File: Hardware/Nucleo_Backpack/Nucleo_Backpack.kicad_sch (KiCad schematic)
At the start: 9 parts, among them J1 CN7, J2 CN10, J4 Conn_01x04

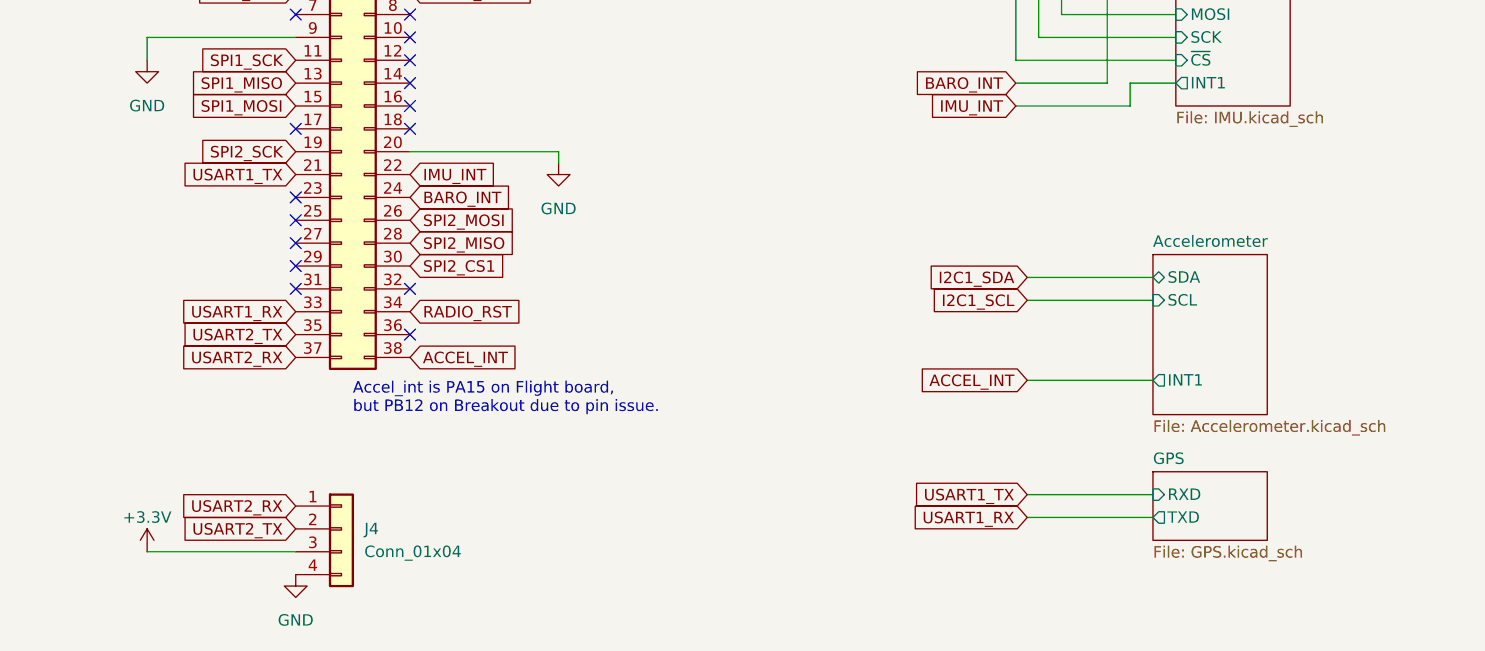
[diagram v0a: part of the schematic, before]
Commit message: Backpack Updates
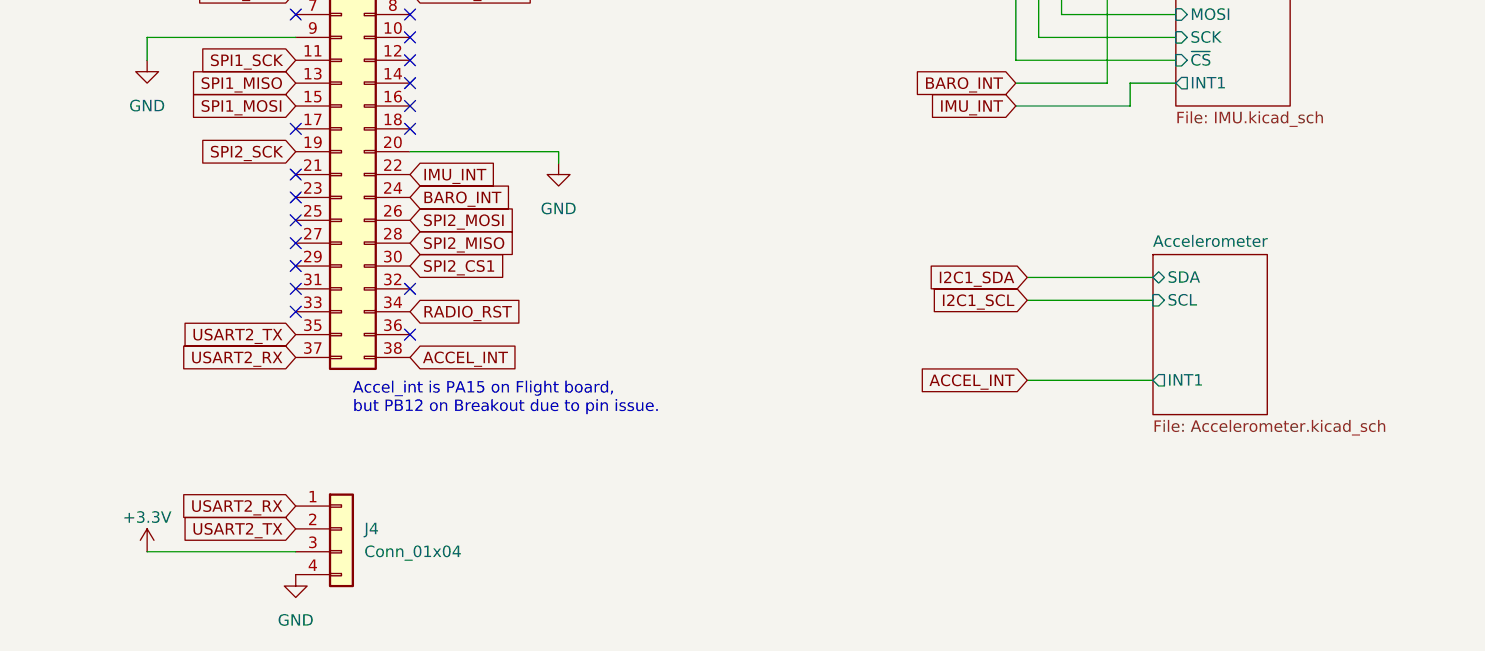
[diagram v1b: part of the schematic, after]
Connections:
- net USART1_RX: no longer names the net of J2.33 (Pin_33)
- net USART1_TX: no longer names the net of J2.21 (Pin_21)
- no-connect marks 39 -> 41
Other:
- removed sheet GPS
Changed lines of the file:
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@@
   (no_connect (at 106.68 110.49))
   (no_connect (at 181.61 91.44))
+  (no_connect (at 168.91 109.22))
   (no_connect (at 106.68 118.11))
   (no_connect (at 106.68 92.71))
@@
   (no_connect (at 181.61 99.06))
   (no_connect (at 181.61 127))
+  (no_connect (at 168.91 124.46))
   (wire (pts (xy 250.19 132.08) (xy 264.16 132.08))
     (stroke (width 0) (type default))
   )
-  (wire (pts (xy 250.19 144.78) (xy 264.16 144.78))
-    (stroke (width 0) (type default))
-  )
   (wire (pts (xy 248.92 73.66) (xy 248.92 96.52))
     (stroke (width 0) (type default))
@@
   )
   (wire (pts (xy 210.82 60.96) (xy 210.82 63.5))
-    (stroke (width 0) (type default))
-  )
-  (wire (pts (xy 250.19 147.32) (xy 264.16 147.32))
     (stroke (width 0) (type default))
   )
@@
     )
   )
-  (global_label "USART1_RX" (shape input) (at 250.19 147.32 180) (fields_autoplaced)
-    (effects (font (size 1.27 1.27)) (justify right))
-    (property "Intersheetrefs" "${INTERSHEET_REFS}" (at 236.5869 147.32 0)
-      (effects (font (size 1.27 1.27)) (justify right) hide)
-    )
-  )
   (global_label "BARO_INT" (shape input) (at 181.61 111.76 0) (fields_autoplaced)
     (effects (font (size 1.27 1.27)) (justify left))
@@
     )
   )
-  (global_label "USART1_TX" (shape input) (at 168.91 109.22 180) (fields_autoplaced)
-    (effects (font (size 1.27 1.27)) (justify right))
-    (property "Intersheetrefs" "${INTERSHEET_REFS}" (at 155.6093 109.22 0)
-      (effects (font (size 1.27 1.27)) (justify right) hide)
-    )
-  )
   (global_label "SPI2_SCK" (shape input) (at 168.91 106.68 180) (fields_autoplaced)
     (effects (font (size 1.27 1.27)) (justify right))
@@
     )
   )
-  (global_label "USART1_TX" (shape input) (at 250.19 144.78 180) (fields_autoplaced)
-    (effects (font (size 1.27 1.27)) (justify right))
-    (property "Intersheetrefs" "${INTERSHEET_REFS}" (at 236.8893 144.78 0)
-      (effects (font (size 1.27 1.27)) (justify right) hide)
-    )
-  )
   (global_label "SDIO_D0" (shape input) (at 181.61 83.82 0) (fields_autoplaced)
     (effects (font (size 1.27 1.27)) (justify left))
@@
     (effects (font (size 1.27 1.27)) (justify right))
     (property "Intersheetrefs" "${INTERSHEET_REFS}" (at 157.0607 86.36 0)
-      (effects (font (size 1.27 1.27)) (justify right) hide)
-    )
-  )
-  (global_label "USART1_RX" (shape input) (at 168.91 124.46 180) (fields_autoplaced)
-    (effects (font (size 1.27 1.27)) (justify right))
-    (property "Intersheetrefs" "${INTERSHEET_REFS}" (at 155.3069 124.46 0)
       (effects (font (size 1.27 1.27)) (justify right) hide)
     )
@@
       )
     )
-  )
-  (sheet (at 264.16 142.24) (size 12.7 7.62) (fields_autoplaced)
-    (stroke (width 0.1524) (type solid))
-    (fill (color 0 0 0 0.0000))
-    (property "Sheetname" "GPS" (at 264.16 141.5284 0)
-      (effects (font (size 1.27 1.27)) (justify left bottom))
-    )
-    (property "Sheetfile" "GPS.kicad_sch" (at 264.16 150.4446 0)
-      (effects (font (size 1.27 1.27)) (justify left top))
-    )
-    (pin "RXD" input (at 264.16 144.78 180)
-      (effects (font (size 1.27 1.27)) (justify left))
-    )
-    (pin "TXD" output (at 264.16 147.32 180)
-      (effects (font (size 1.27 1.27)) (justify left))
-    )
-    (instances
-      (project "Nucleo_Backpack"
-        (path "/e8eb85d5-f1ff-4500-895d-25b9ff5f6d36" (page "5"))
-      )
-    )
